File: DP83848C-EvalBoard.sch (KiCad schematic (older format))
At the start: 4 parts

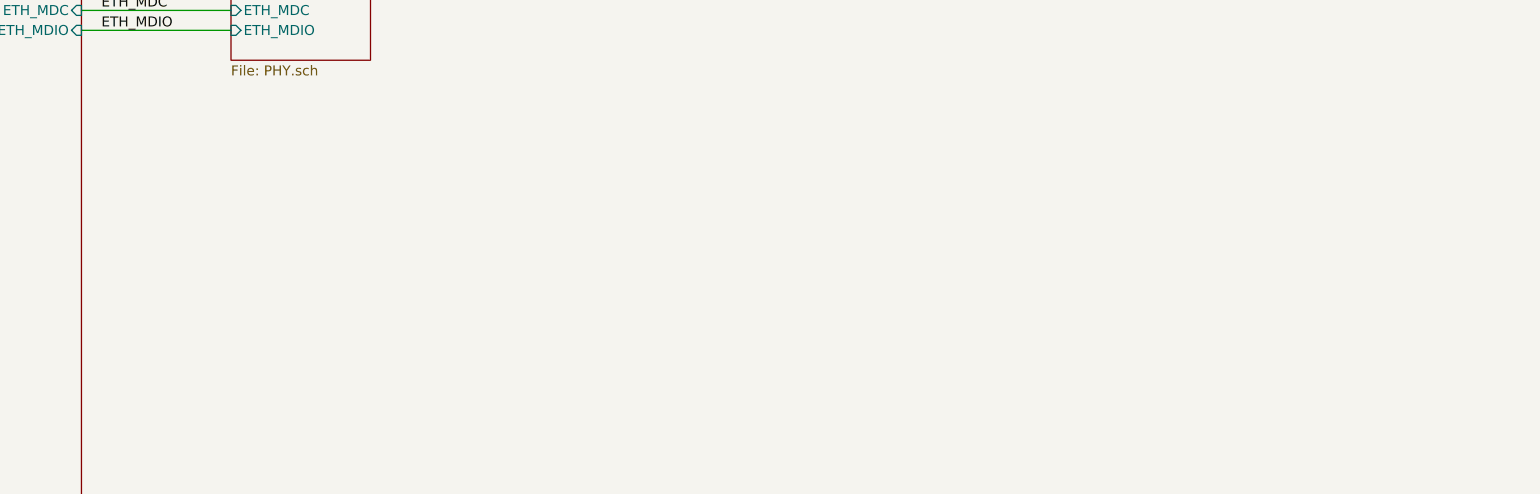
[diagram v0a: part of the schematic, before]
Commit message: Firmware
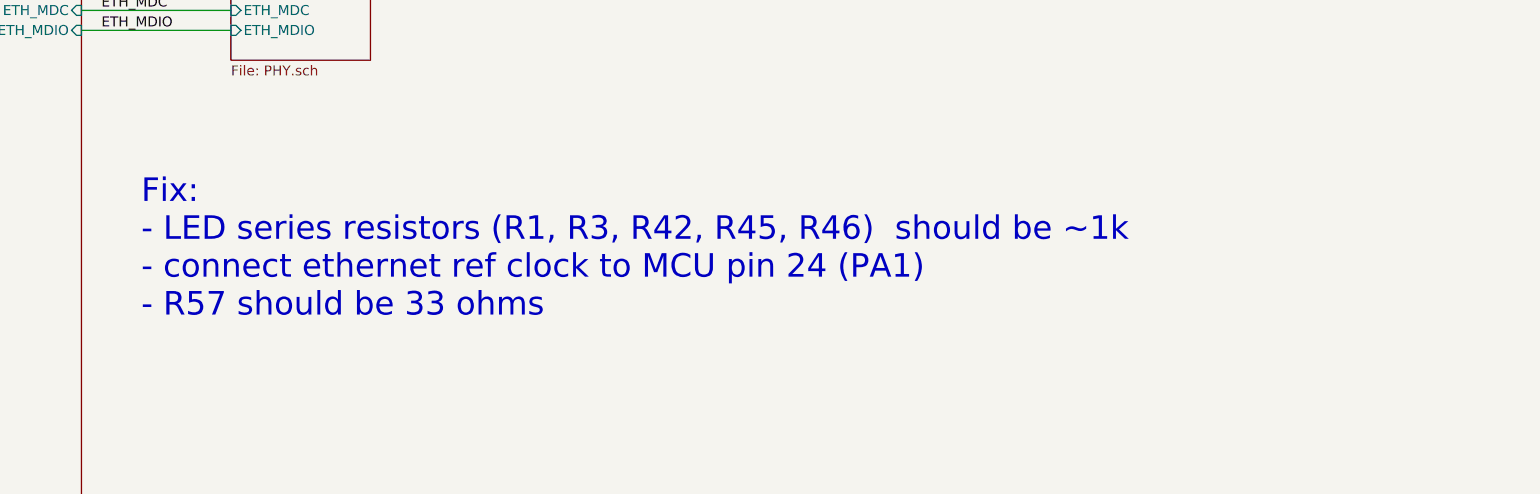
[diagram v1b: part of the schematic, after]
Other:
- note added: "Fix:\n- LED series resistors (R1, R3, R42, R45, R46) should be ~~1k\n- connect ethernet ref clock to MCU pin 24 (PA1)\n- R57 should be 33 ohms"
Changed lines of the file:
@@
 	1    0    0    -1
 $EndComp
+Text Notes 5300 4200 0    118  ~ 0
+Fix:\n- LED series resistors (R1, R3, R42, R45, R46)  should be ~~1k\n- connect ethernet ref clock to MCU pin 24 (PA1)\n- R57 should be 33 ohms
 $EndSCHEMATC
